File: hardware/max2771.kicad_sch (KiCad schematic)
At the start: 23 parts, among them IC7 MAX2771ETI+

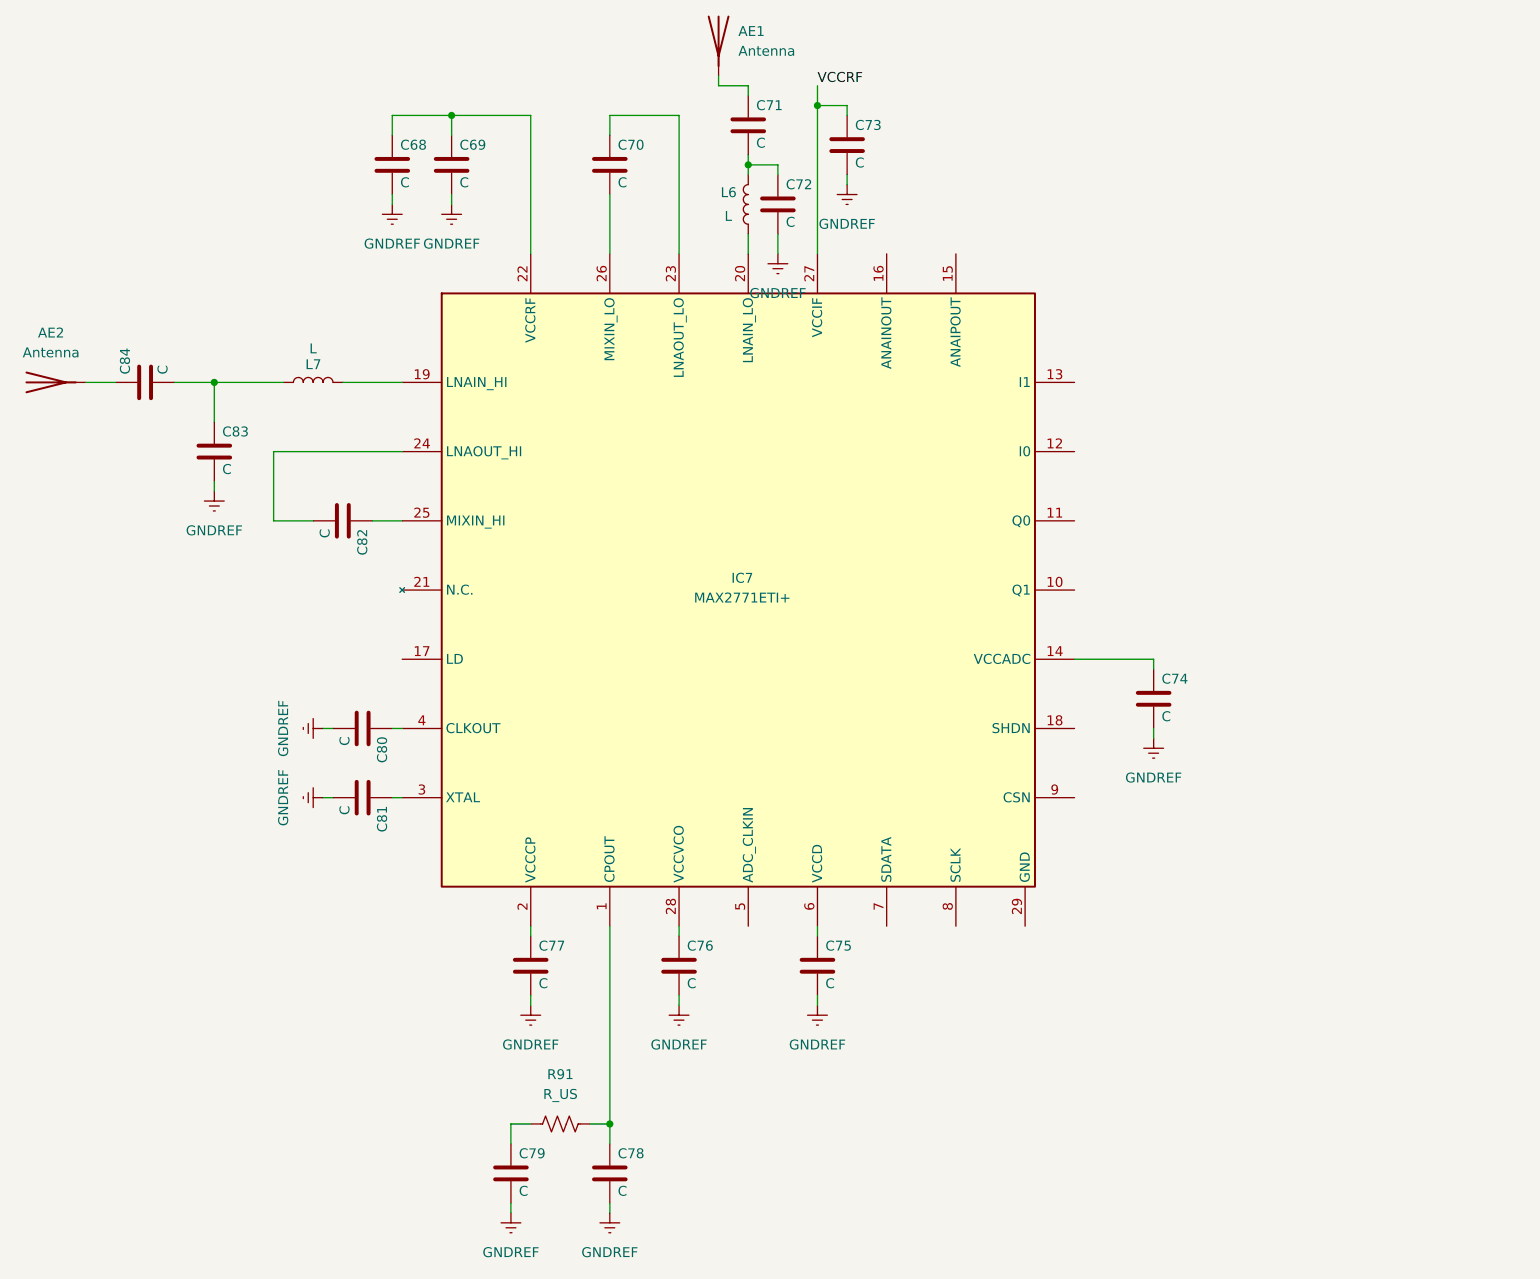
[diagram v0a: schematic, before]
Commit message: updated schematic
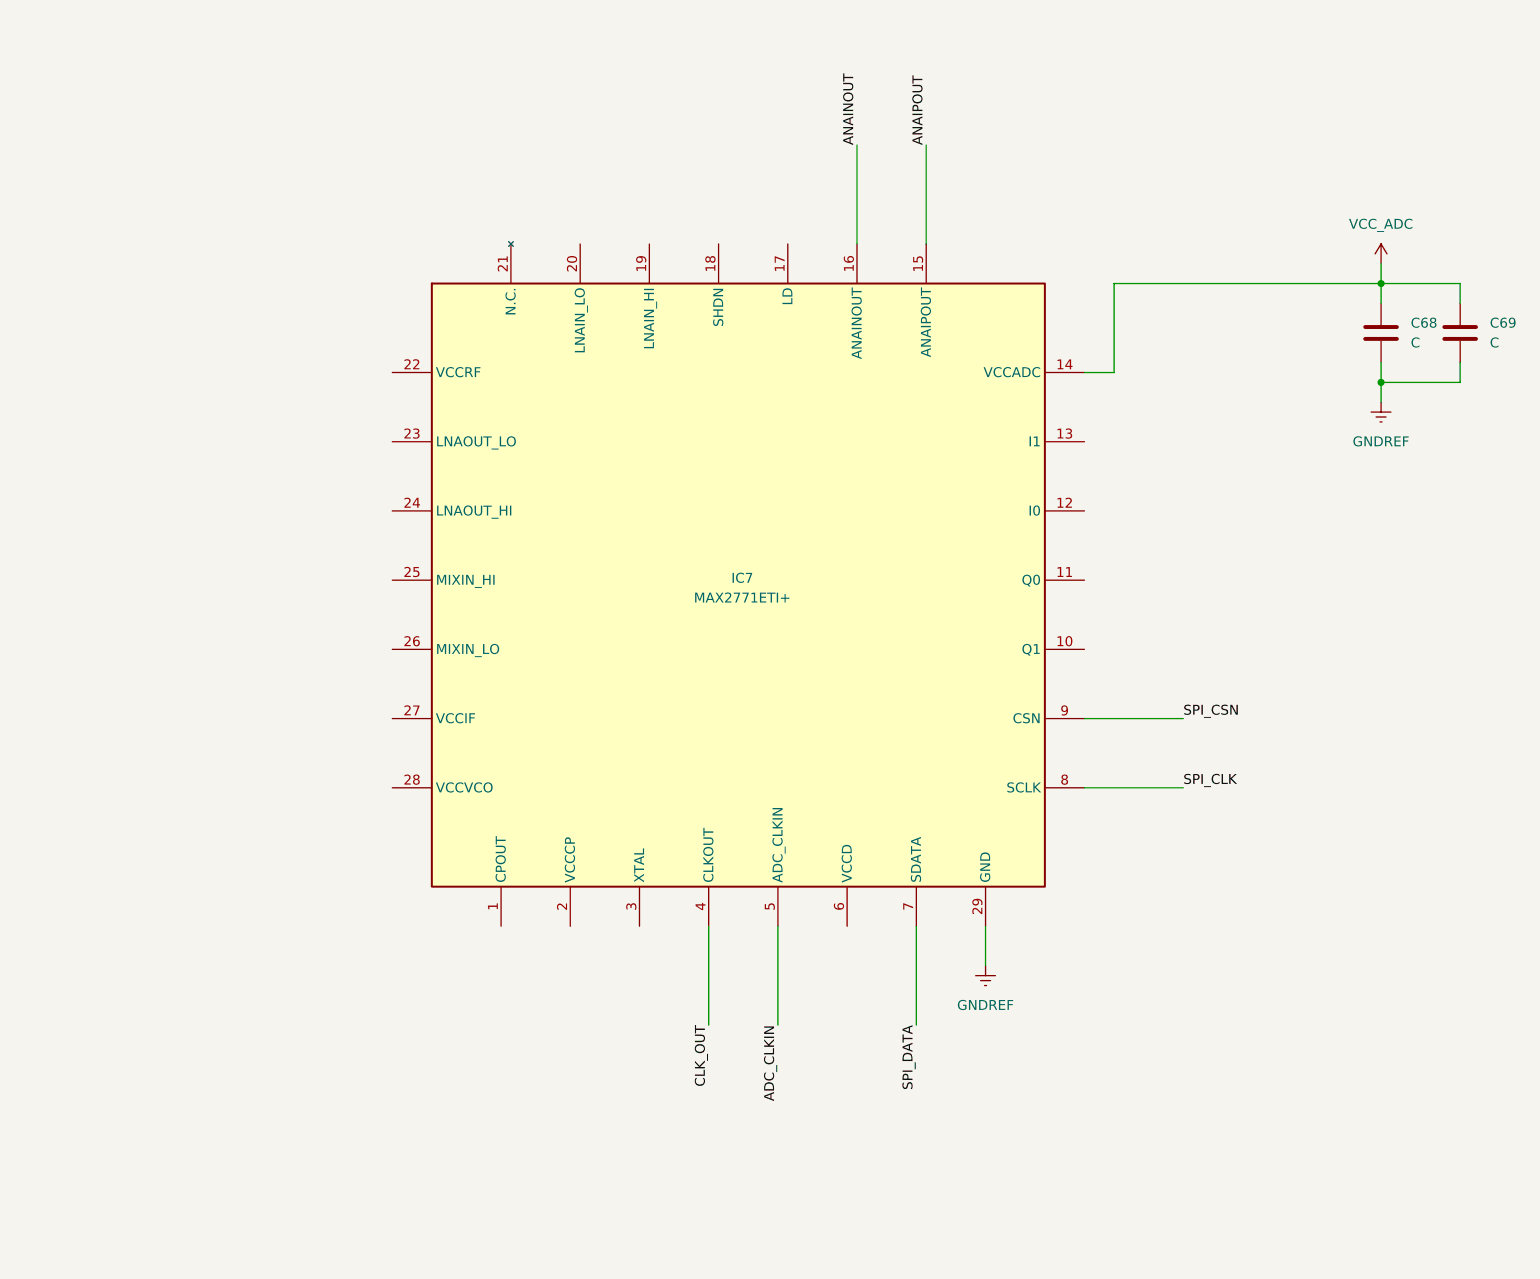
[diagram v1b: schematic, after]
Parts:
- removed AE1, AE2: Antenna, symbol Device:Antenna
- removed C70, C71, C72, C73, C74, C75, C76, C77, C78, C79, C80, C81, C82, C83, C84: C, symbol Device:C
- removed L6, L7: L, symbol Device:L
- removed R91: R_US, symbol Device:R_US
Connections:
- net GNDREF: now also C68.2, C69.2, IC7.29 (GND); no longer C68.1, C69.1
- net VCC_ADC: now reaches IC7.14 (VCCADC)
- net VCC_ADC: now also C68.1, C69.1
- net ANAIPOUT: now reaches IC7.15 (ANAIPOUT)
- net ANAINOUT: now reaches IC7.16 (ANAINOUT)
- net CLK_OUT: now reaches IC7.4 (CLKOUT)
- net ADC_CLKIN: now reaches IC7.5 (ADC_CLKIN)
- net SPI_DATA: now reaches IC7.7 (SDATA)
- net SPI_CLK: now reaches IC7.8 (SCLK)
- net SPI_CSN: now reaches IC7.9 (CSN)
- net VCCRF: no longer names the net of IC7.27 (VCCIF)
- now unconnected: IC7.22 (VCCRF)
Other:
- moved on the sheet: IC7
